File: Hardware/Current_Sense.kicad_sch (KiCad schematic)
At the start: 32 parts, among them IC2 INA241A4IDR, IC3 AMC1350DWVR, IC4 TLV9002QDRQ1, J6 Scrut Conn, SW3 Scrut Select, U9 REF35125QDBVR

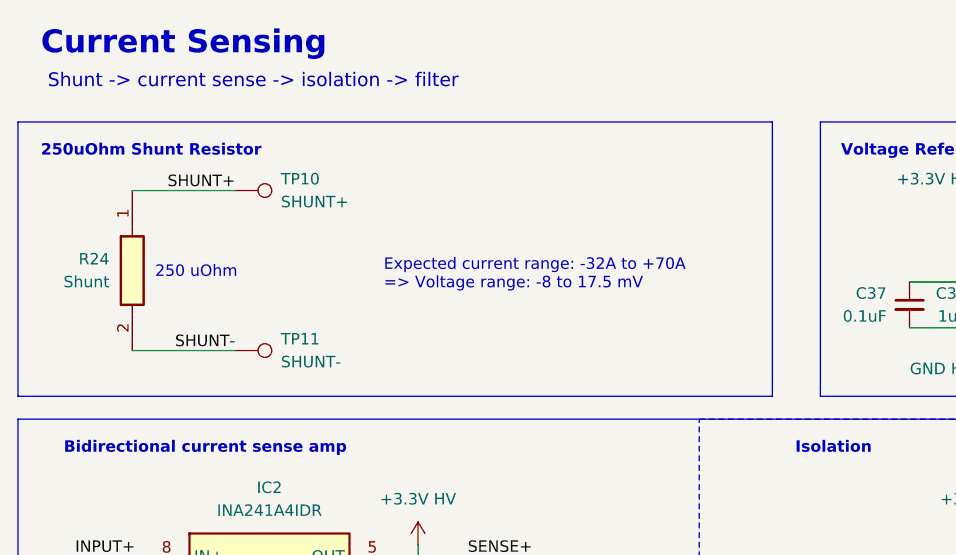
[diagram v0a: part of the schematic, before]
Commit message: changed shunt model, moved around folders; initial layout, routing soon
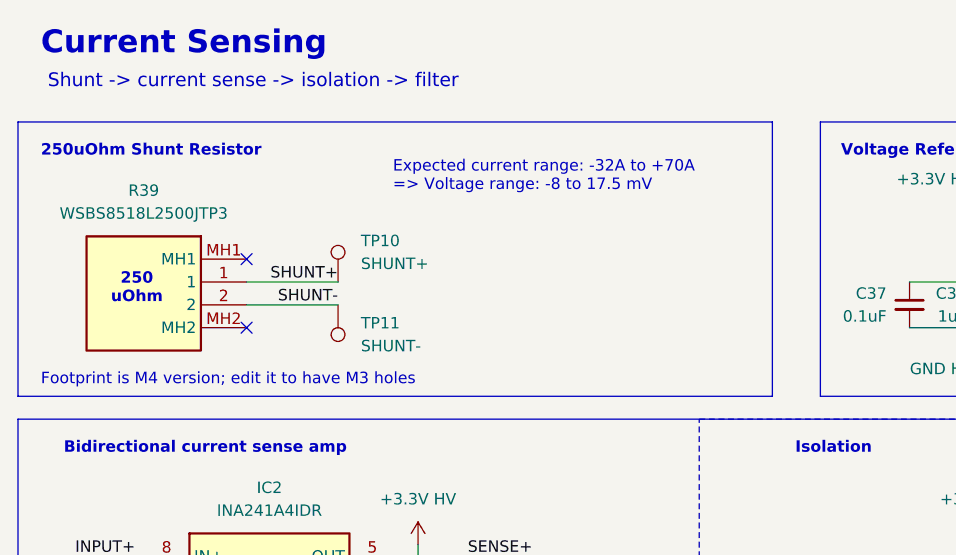
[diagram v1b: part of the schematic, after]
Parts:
- removed R24: Shunt, Parts:WSBS8518L2500JK, symbol WSBS8518L2500JK:WSBS8518L2500JK
- added R39: WSBS8518L2500JTP3, WSBS8518L2500JKM4, symbol WSBS8518L2500JKM4:WSBS8518L2500JKM4
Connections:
- net SHUNT+: now also R39.1
- net SHUNT-: now also R39.2
- no-connect marks 1 -> 3
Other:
- note added: "Footprint is M4 version; edit it to have M3 holes"
- moved on the sheet: TP10, TP11
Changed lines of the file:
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@@
 		)
 	)
-	(text "250 uOhm"
+	(text "250 \nuOhm"
 		(exclude_from_sim no)
-		(at 35.052 44.704 0)
+		(at 28.448 46.482 0)
 		(effects
 			(font
 				(size 1.27 1.27)
+				(thickness 0.254)
+				(bold yes)
 			)
 		)
@@
 	(text "Expected current range: -32A to +70A\n=> Voltage range: -8 to 17.5 mV"
 		(exclude_from_sim no)
-		(at 55.88 43.18 0)
+		(at 56.896 32.258 0)
 		(effects
 			(font
@@
 		)
 	)
+	(text "Footprint is M4 version; edit it to have M3 holes"
+		(exclude_from_sim no)
+		(at 17.78 55.88 0)
+		(effects
+			(font
+				(size 1.27 1.27)
+				(color 255 8 29 1)
+			)
+			(justify left top)
+		)
+	)
 	(junction
 		(at 29.21 154.94)
@@
 		(at 138.43 46.99)
 	)
+	(no_connect
+		(at 40.64 43.18)
+	)
+	(no_connect
+		(at 40.64 50.8)
+	)
 	(wire
 		(pts
@@
 	(wire
 		(pts
-			(xy 27.94 35.56) (xy 39.37 35.56)
+			(xy 40.64 45.72) (xy 50.8 45.72)
 		)
 		(stroke
@@
 	(wire
 		(pts
-			(xy 27.94 53.34) (xy 39.37 53.34)
+			(xy 40.64 48.26) (xy 50.8 48.26)
 		)
 		(stroke
@@
 	)
 	(label "SHUNT-"
-		(at 39.37 53.34 180)
+		(at 50.8 48.26 180)
 		(effects
 			(font
@@
 	)
 	(label "SHUNT+"
-		(at 39.37 35.56 180)
+		(at 50.8 45.72 180)
 		(effects
 			(font
@@
 	)
 	(symbol
+		(lib_id "WSBS8518L2500JKM4:WSBS8518L2500JKM4")
+		(at 40.64 43.18 0)
+		(mirror y)
+		(unit 1)
+		(exclude_from_sim no)
+		(in_bom yes)
+		(on_board yes)
+		(dnp no)
+		(fields_autoplaced yes)
+		(property "Reference" "R39"
+			(at 29.21 35.56 0)
+			(effects
+				(font
+					(size 1.27 1.27)
+				)
+			)
+		)
+		(property "Value" "WSBS8518L2500JTP3"
+			(at 29.21 38.1 0)
+			(effects
+				(font
+					(size 1.27 1.27)
+				)
+			)
+		)
+		(property "Footprint" "WSBS8518L2500JKM4"
+			(at 21.59 138.1 0)
+			(effects
+				(font
+					(size 1.27 1.27)
+				)
+				(justify left top)
+				(hide yes)
+			)
+		)
+		(property "Datasheet" "https://www.vishay.com/docs/30392/wsbs8518p3.pdf"
+			(at 21.59 238.1 0)
+			(effects
+				(font
+					(size 1.27 1.27)
+				)
+				(justify left top)
+				(hide yes)
+			)
+		)
+		(property "Description" "Power Metal Strip Battery Shunt Resistor With M4 Tapped Holes Very Low Value (50 u, 100 u, 125 u, and 250 u)"
+			(at 40.64 43.18 0)
+			(effects
+				(font
+					(size 1.27 1.27)
+				)
+				(hide yes)
+			)
+		)
+		(property "Height" "3"
+			(at 21.59 438.1 0)
+			(effects
+				(font
+					(size 1.27 1.27)
+				)
+				(justify left top)
+				(hide yes)
+			)
+		)
+		(property "Mouser Part Number" "71-WSBS8518L2500JTP3"
+			(at 21.59 538.1 0)
+			(effects
+				(font
+					(size 1.27 1.27)
+				)
+				(justify left top)
+				(hide yes)
+			)
+		)
+		(property "Mouser Price/Stock" "https://www.mouser.co.uk/ProductDetail/Vishay-Dale/WSBS8518L2500JKM4?qs=BZBei1rCqCBDT%2FHsm0OnWA%3D%3D"
+			(at 21.59 638.1 0)
+			(effects
+				(font
+					(size 1.27 1.27)
+				)
+				(justify left top)
+				(hide yes)
+			)
+		)
+		(property "Manufacturer_Name" "Vishay"
+			(at 21.59 738.1 0)
+			(effects
+				(font
+					(size 1.27 1.27)
+				)
+				(justify left top)
+				(hide yes)
+			)
+		)
+		(property "Manufacturer_Part_Number" "WSBS8518L2500JTP3"
+			(at 21.59 838.1 0)
+			(effects
+				(font
+					(size 1.27 1.27)
+				)
+				(justify left top)
+				(hide yes)
+			)
+		)
+		(pin "1"
+		)
+		(pin "MH2"
+		)
+		(pin "MH1"
+		)
+		(pin "2"
+		)
+		(instances
+			(project ""
+				(path "/a452d214-ea00-440d-a445-5d6103fda43a/7e38ba4d-a54c-4f69-a074-7d0a3dae713a"
+					(reference "R39")
+					(unit 1)
+				)
+			)
+		)
+	)
+	(symbol
 		(lib_id "Device:C_Small")
 		(at 114.3 82.55 0)
@@
 	(symbol
 		(lib_id "Connector:TestPoint")
-		(at 39.37 35.56 270)
+		(at 50.8 45.72 0)
 		(unit 1)
 		(exclude_from_sim no)
@@
 		(fields_autoplaced yes)
 		(property "Reference" "TP10"
-			(at 44.45 34.2899 90)
+			(at 53.34 41.1479 0)
 			(effects
 				(font
@@
 		)
 		(property "Value" "SHUNT+"
-			(at 44.45 36.8299 90)
+			(at 53.34 43.6879 0)
 			(effects
 				(font
@@
 		)
 		(property "Footprint" "TestPoint:TestPoint_Pad_1.0x1.0mm"
-			(at 39.37 40.64 0)
+			(at 55.88 45.72 0)
 			(effects
 				(font
@@
 		)
 		(property "Datasheet" "~"
-			(at 39.37 40.64 0)
+			(at 55.88 45.72 0)
 			(effects
 				(font
@@
 		)
 		(property "Description" "test point"
-			(at 39.37 35.56 0)
+			(at 50.8 45.72 0)
 			(effects
 				(font
@@
 	)
 	(symbol
-		(lib_id "WSBS8518L2500JK:WSBS8518L2500JK")
-		(at 27.94 35.56 90)
-		(mirror x)
-		(unit 1)
-		(exclude_from_sim no)
-		(in_bom yes)
-		(on_board yes)
-		(dnp no)
-		(property "Reference" "R24"
-			(at 25.4 43.1799 90)
-			(effects
-				(font
-					(size 1.27 1.27)
-				)
-				(justify left)
-			)
-		)
-		(property "Value" "Shunt"
-			(at 25.4 45.7199 90)
-			(effects
-				(font
-					(size 1.27 1.27)
-				)
-				(justify left)
-			)
-		)
-		(property "Footprint" "Parts:WSBS8518L2500JK"
-			(at 124.13 49.53 0)
-			(effects
-				(font
-					(size 1.27 1.27)
-				)
-				(justify left top)
-				(hide yes)
-			)
-		)
-		(property "Datasheet" "https://www.vishay.com/docs/30134/wsbs8518.pdf"
-			(at 224.13 49.53 0)
-			(effects
-				(font
-					(size 1.27 1.27)
-				)
-				(justify left top)
-				(hide yes)
-			)
-		)
-		(property "Description" "Current Sense Resistors - Through Hole 36watt 250 micro-ohm 5% Battery Shunt"
-			(at 27.94 35.56 0)
-			(effects
-				(font
-					(size 1.27 1.27)
-				)
-				(hide yes)
-			)
-		)
-		(property "Height" "3.1"
-			(at 424.13 49.53 0)
-			(effects
-				(font
-					(size 1.27 1.27)
-				)
-				(justify left top)
-				(hide yes)
-			)
-		)
-		(property "Mouser Part Number" "71-WSBS8518L2500JK"
-			(at 524.13 49.53 0)
-			(effects
-				(font
-					(size 1.27 1.27)
-				)
-				(justify left top)
-				(hide yes)
-			)
-		)
-		(property "Mouser Price/Stock" "https://www.mouser.co.uk/ProductDetail/Vishay-Dale/WSBS8518L2500JK?qs=i2mp%2Fn9EmlJ0b%2F4LBxCPeA%3D%3D"
-			(at 624.13 49.53 0)
-			(effects
-				(font
-					(size 1.27 1.27)
-				)
-				(justify left top)
-				(hide yes)
-			)
-		)
-		(property "Manufacturer_Name" "Vishay"
-			(at 724.13 49.53 0)
-			(effects
-				(font
-					(size 1.27 1.27)
-				)
-				(justify left top)
-				(hide yes)
-			)
-		)
-		(property "Manufacturer_Part_Number" "WSBS8518L2500JK"
-			(at 824.13 49.53 0)
-			(effects
-				(font
-					(size 1.27 1.27)
-				)
-				(justify left top)
-				(hide yes)
-			)
-		)
-		(pin "1"
-		)
-		(pin "2"
-		)
-		(instances
-			(project ""
-				(path "/a452d214-ea00-440d-a445-5d6103fda43a/7e38ba4d-a54c-4f69-a074-7d0a3dae713a"
-					(reference "R24")
-					(unit 1)
-				)
-			)
-		)
-	)
-	(symbol
 		(lib_id "Device:C_Small")
 		(at 154.94 90.17 0)
@@
 	(symbol
 		(lib_id "Connector:TestPoint")
-		(at 39.37 53.34 270)
+		(at 50.8 48.26 180)
 		(unit 1)
 		(exclude_from_sim no)
@@
 		(fields_autoplaced yes)
 		(property "Reference" "TP11"
-			(at 44.45 52.0699 90)
+			(at 53.34 50.2919 0)
 			(effects
 				(font
 					(size 1.27 1.27)
 				)
-				(justify left)
+				(justify right)
 			)
 		)
 		(property "Value" "SHUNT-"
-			(at 44.45 54.6099 90)
+			(at 53.34 52.8319 0)
 			(effects
 				(font
 					(size 1.27 1.27)
 				)
-				(justify left)
+				(justify right)
 			)
 		)
 		(property "Footprint" "TestPoint:TestPoint_Pad_1.0x1.0mm"
-			(at 39.37 58.42 0)
+			(at 45.72 48.26 0)
 			(effects
 				(font
@@
 		)
 		(property "Datasheet" "~"
-			(at 39.37 58.42 0)
+			(at 45.72 48.26 0)
 			(effects
 				(font
@@
 		)
 		(property "Description" "test point"
-			(at 39.37 53.34 0)
+			(at 50.8 48.26 0)
 			(effects
 				(font

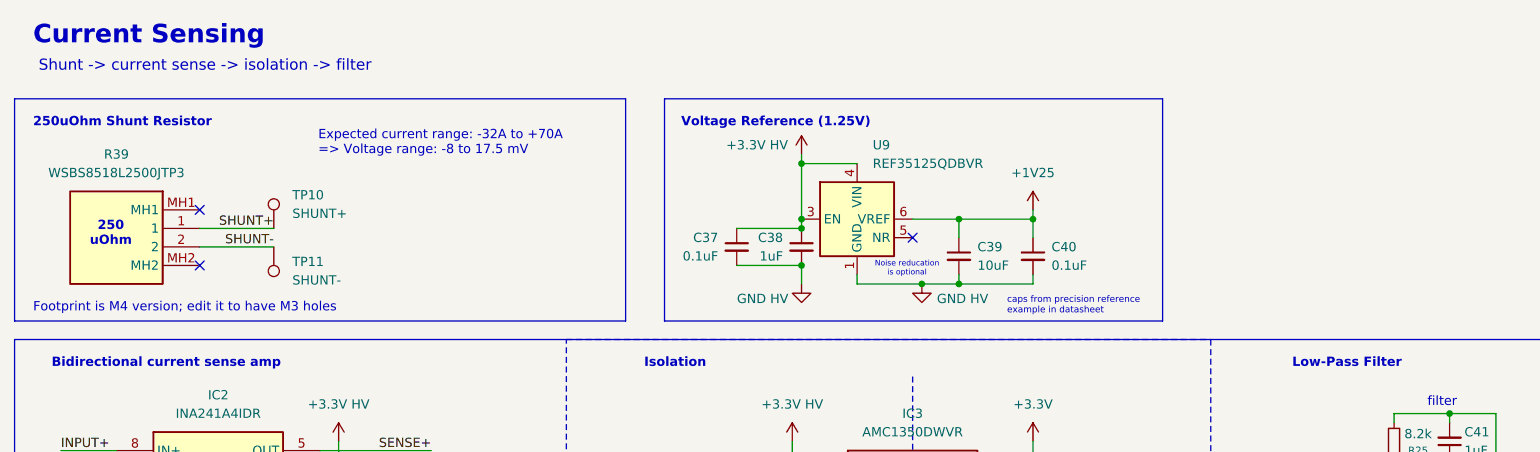
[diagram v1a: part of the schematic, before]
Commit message: 9/20 workday: some layout stuff ye ye
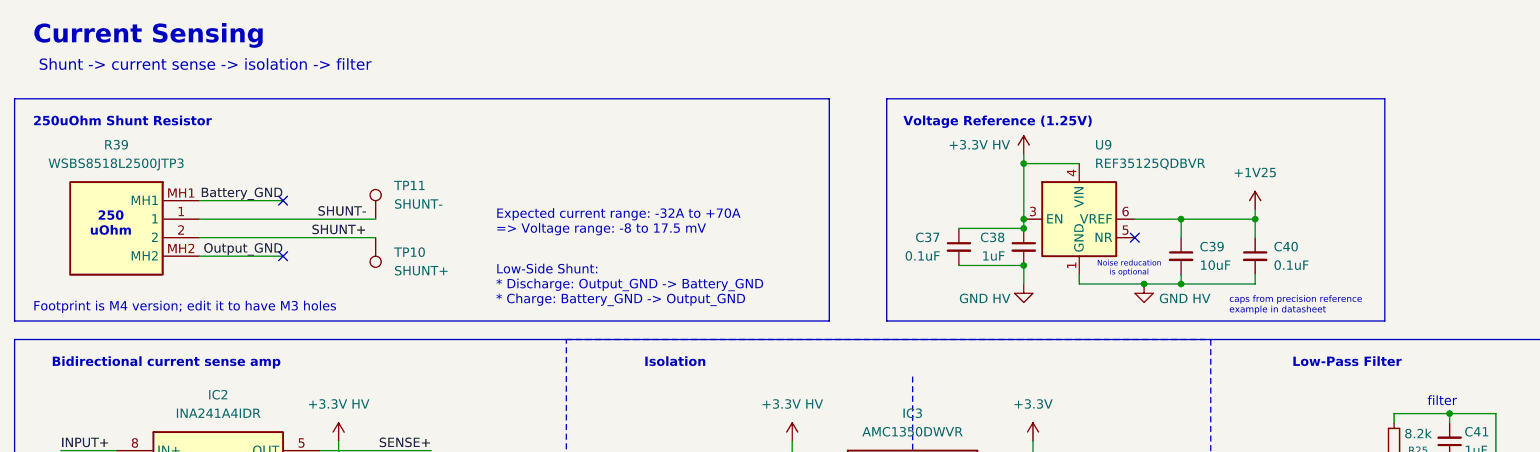
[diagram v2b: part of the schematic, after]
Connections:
- net SHUNT+: now also R39.2; no longer R39.1
- net SHUNT-: now also R39.1; no longer R39.2
- net Battery_GND: now reaches R39.MH1
- net Output_GND: now reaches R39.MH2
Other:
- note added: "Low-Side Shunt: * Discharge: Output_GND -> Battery_GND * Charge: Battery_GND -> Output_GND"
- moved on the sheet: C37, C38, C39, C40, R39, TP10, TP11, U9
